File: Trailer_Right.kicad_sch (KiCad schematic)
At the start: 11 parts, among them Q28 IRLZ44N, SW5 SW_SPST, U8 LM339

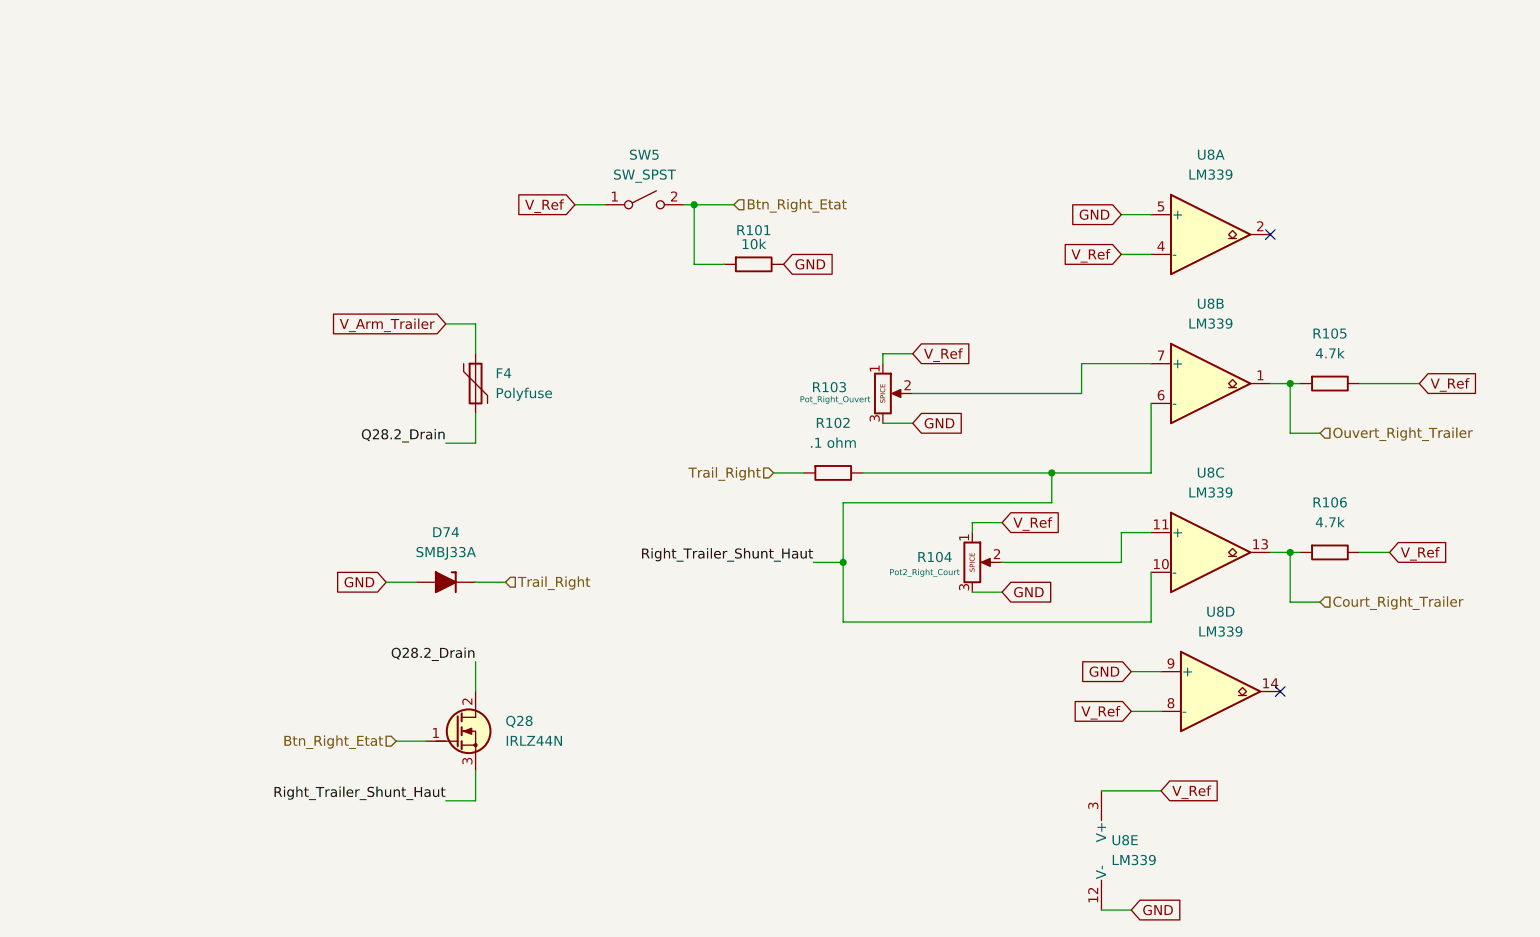
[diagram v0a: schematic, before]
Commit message: Add files via upload
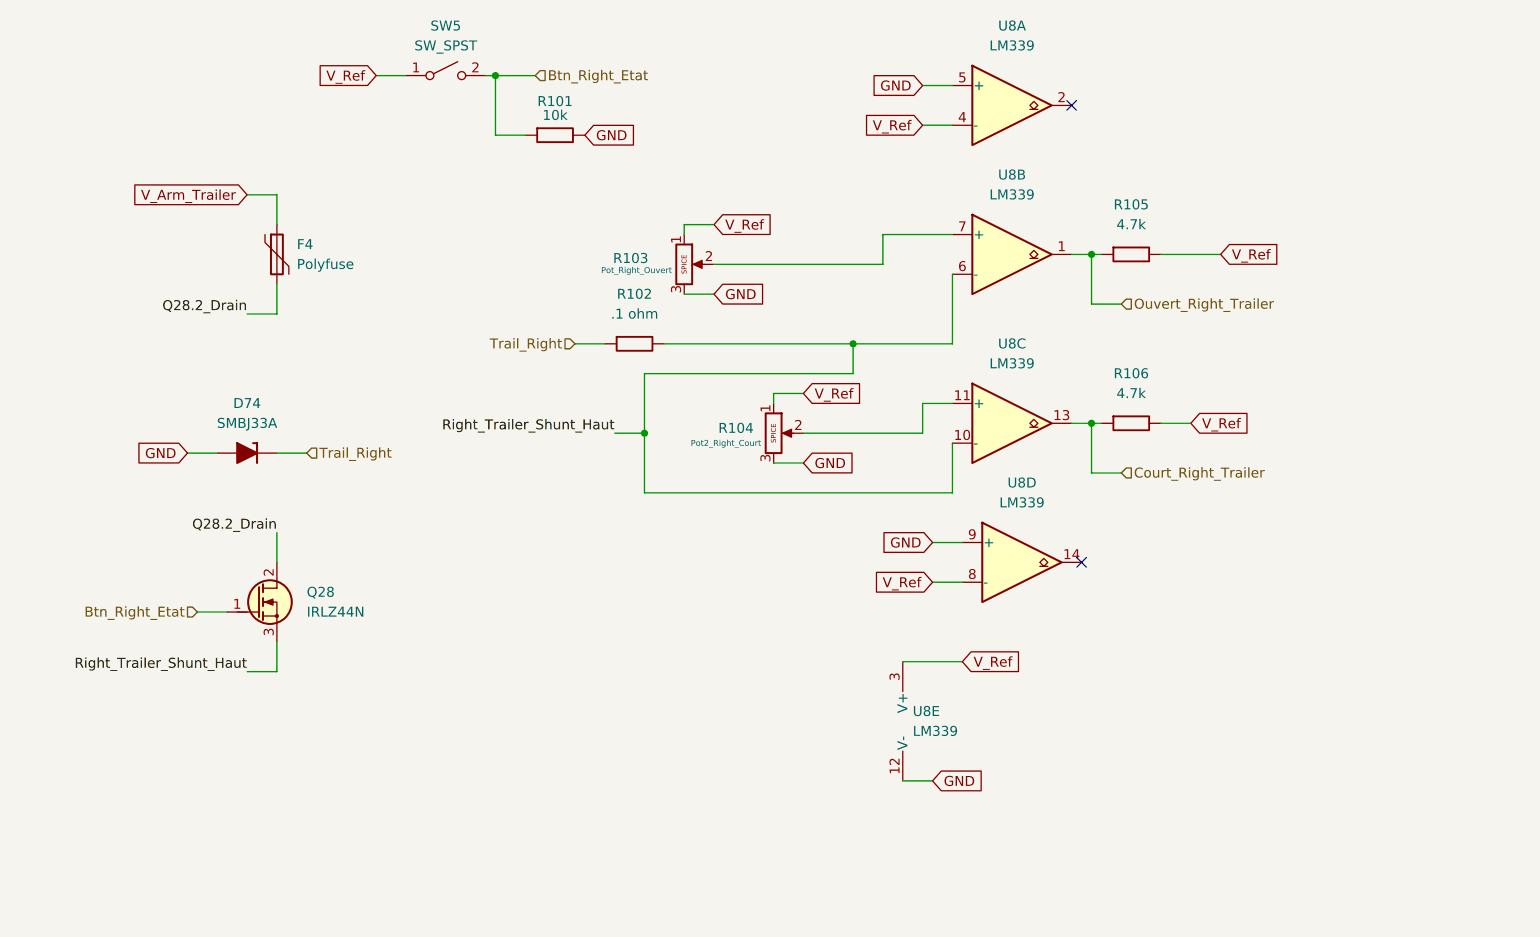
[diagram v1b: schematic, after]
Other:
- moved on the sheet: D74, F4, Q28, R101, R102, R103, R104, R105, R106, SW5, U8A, U8B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

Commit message: Add files via upload
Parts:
- R102: footprint Resistor_THT:R_Axial_DIN0207_L6.3mm_D2.5mm_P10.16mm_Horizontal -> PCM_SL_Devices:Resistor_5W
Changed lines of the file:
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@@
 			)
 		)
-		(property "Footprint" "Resistor_THT:R_Axial_DIN0207_L6.3mm_D2.5mm_P10.16mm_Horizontal"
+		(property "Footprint" "PCM_SL_Devices:Resistor_5W"
 			(at 93.599 65.278 0)
 			(hide yes)

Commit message: Add files via upload
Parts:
- R102: footprint PCM_SL_Devices:Resistor_5W -> Resistor_THT:R_Axial_Power_L25.0mm_W9.0mm_P27.94mm
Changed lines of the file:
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@@
 			)
 		)
-		(property "Footprint" "PCM_SL_Devices:Resistor_5W"
+		(property "Footprint" "Resistor_THT:R_Axial_Power_L25.0mm_W9.0mm_P27.94mm"
 			(at 93.599 65.278 0)
 			(hide yes)

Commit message: Add files via upload
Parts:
- R103, R104: footprint (none) -> TRIM_3296W1103LF:TRIM_3296W1103LF
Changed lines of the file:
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@@
 			)
 		)
-		(property "Footprint" ""
+		(property "Footprint" "TRIM_3296W1103LF:TRIM_3296W1103LF"
 			(at 99.06 50.8 0)
 			(hide yes)
@@
 			)
 		)
-		(property "Footprint" ""
+		(property "Footprint" "TRIM_3296W1103LF:TRIM_3296W1103LF"
 			(at 110.49 72.39 0)
 			(hide yes)

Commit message: Add files via upload
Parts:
- U8: footprint (none) -> Package_DIP:DIP-14_W7.62mm_Socket
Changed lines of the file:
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@@
 			)
 		)
-		(property "Footprint" ""
+		(property "Footprint" "Package_DIP:DIP-14_W7.62mm_Socket"
 			(at 139.7 68.58 0)
 			(hide yes)
@@
 			)
 		)
-		(property "Footprint" ""
+		(property "Footprint" "Package_DIP:DIP-14_W7.62mm_Socket"
 			(at 139.7 27.94 0)
 			(hide yes)
@@
 			)
 		)
-		(property "Footprint" ""
+		(property "Footprint" "Package_DIP:DIP-14_W7.62mm_Socket"
 			(at 128.27 106.68 0)
 			(hide yes)
@@
 			)
 		)
-		(property "Footprint" ""
+		(property "Footprint" "Package_DIP:DIP-14_W7.62mm_Socket"
 			(at 139.7 46.99 0)
 			(hide yes)
@@
 			)
 		)
-		(property "Footprint" ""
+		(property "Footprint" "Package_DIP:DIP-14_W7.62mm_Socket"
 			(at 140.97 86.36 0)
 			(hide yes)

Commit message: Add files via upload
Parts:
- U8: footprint Package_DIP:DIP-14_W7.62mm_Socket -> (none)
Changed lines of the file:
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@@
 			)
 		)
-		(property "Footprint" "Package_DIP:DIP-14_W7.62mm_Socket"
+		(property "Footprint" ""
 			(at 139.7 68.58 0)
 			(hide yes)
@@
 			)
 		)
-		(property "Footprint" "Package_DIP:DIP-14_W7.62mm_Socket"
+		(property "Footprint" ""
 			(at 139.7 27.94 0)
 			(hide yes)
@@
 			)
 		)
-		(property "Footprint" "Package_DIP:DIP-14_W7.62mm_Socket"
+		(property "Footprint" ""
 			(at 128.27 106.68 0)
 			(hide yes)
@@
 			)
 		)
-		(property "Footprint" "Package_DIP:DIP-14_W7.62mm_Socket"
+		(property "Footprint" ""
 			(at 139.7 46.99 0)
 			(hide yes)
@@
 			)
 		)
-		(property "Footprint" "Package_DIP:DIP-14_W7.62mm_Socket"
+		(property "Footprint" ""
 			(at 140.97 86.36 0)
 			(hide yes)

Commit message: Add files via upload
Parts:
- R102: footprint Resistor_THT:R_Axial_Power_L25.0mm_W9.0mm_P27.94mm -> Resistor_THT:R_Axial_DIN0207_L6.3mm_D2.5mm_P10.16mm_Horizontal
- R103, R104: footprint TRIM_3296W1103LF:TRIM_3296W1103LF -> (none)
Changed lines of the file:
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@@
 			)
 		)
-		(property "Footprint" "TRIM_3296W1103LF:TRIM_3296W1103LF"
+		(property "Footprint" ""
 			(at 99.06 50.8 0)
 			(hide yes)
@@
 			)
 		)
-		(property "Footprint" "TRIM_3296W1103LF:TRIM_3296W1103LF"
+		(property "Footprint" ""
 			(at 110.49 72.39 0)
 			(hide yes)
@@
 			)
 		)
-		(property "Footprint" "Resistor_THT:R_Axial_Power_L25.0mm_W9.0mm_P27.94mm"
+		(property "Footprint" "Resistor_THT:R_Axial_DIN0207_L6.3mm_D2.5mm_P10.16mm_Horizontal"
 			(at 93.599 65.278 0)
 			(hide yes)
